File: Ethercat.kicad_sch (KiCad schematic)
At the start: 51 parts, among them J1 RJ45_Amphenol_RJMG1BD3B8K1ANR, J2 RJ45_Amphenol_RJMG1BD3B8K1ANR, Y1 25Mhz

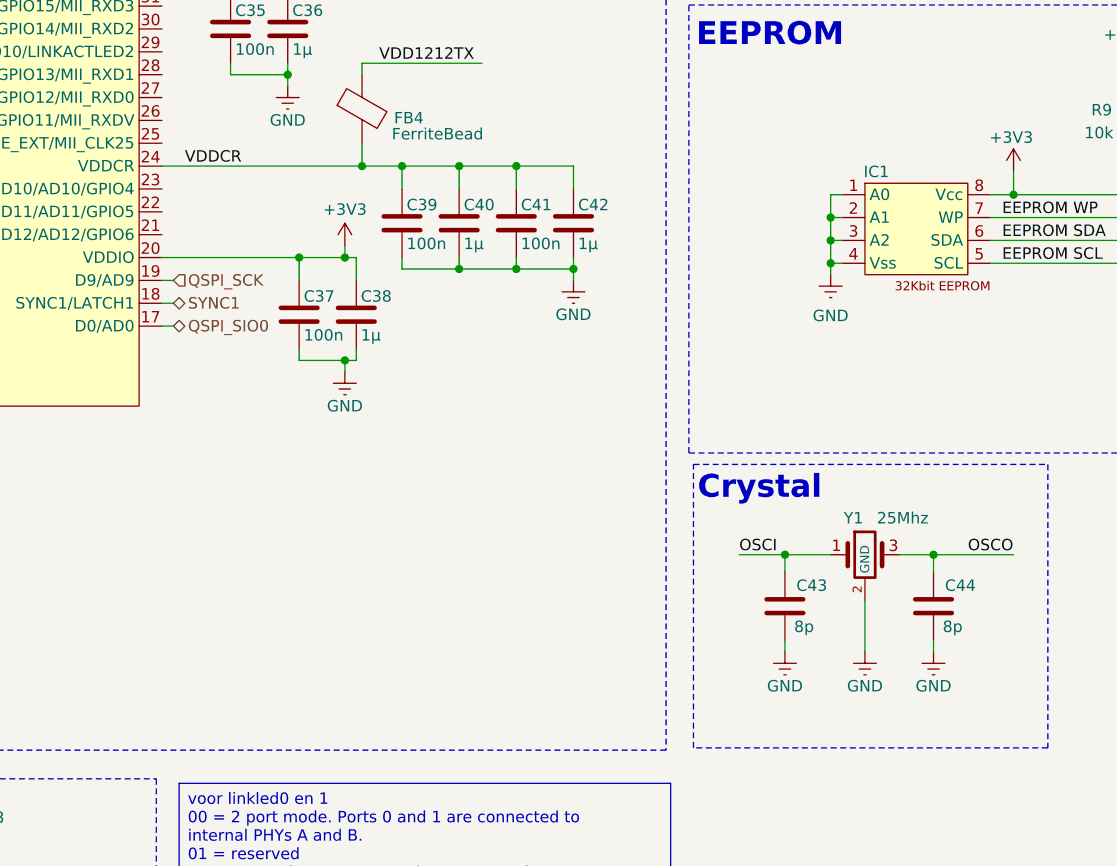
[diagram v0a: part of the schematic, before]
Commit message: al de main blokken bij elkaar gezet op juiste plaats
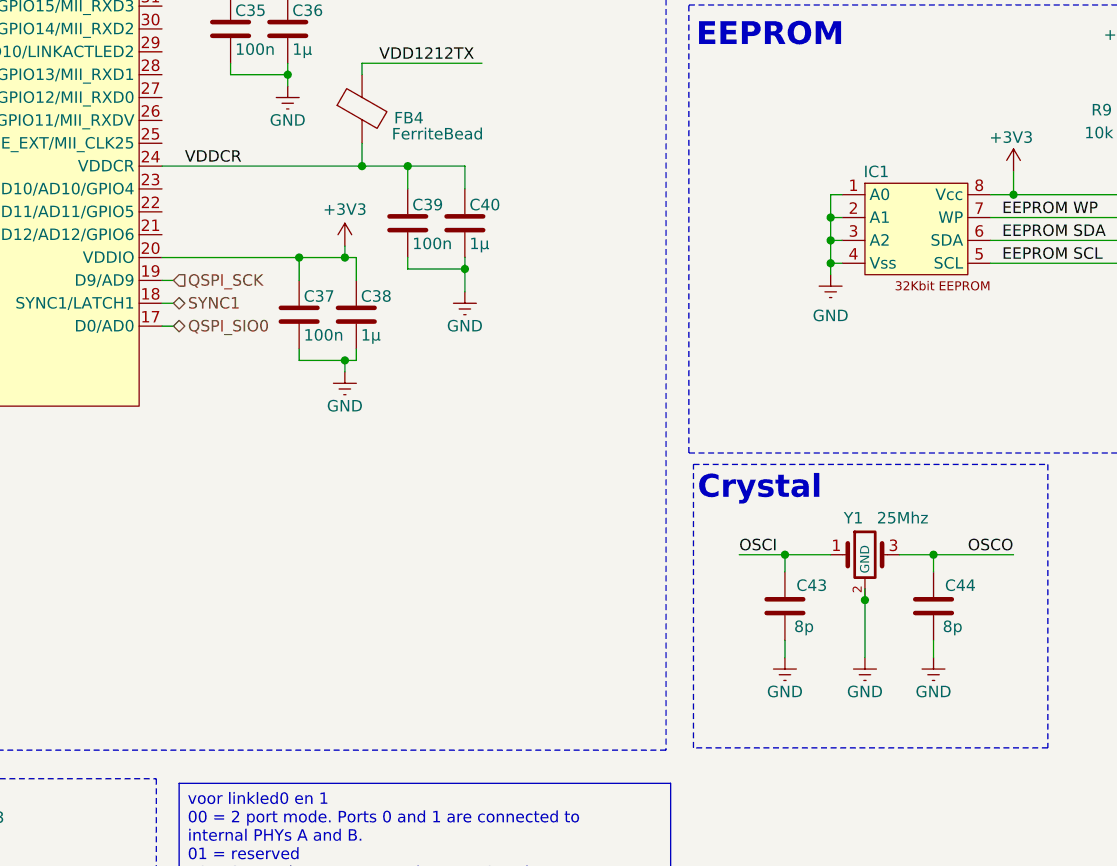
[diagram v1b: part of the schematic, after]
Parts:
- removed C41: 100n, Capacitor_SMD:C_0603_1608Metric, symbol Device:C
- removed C42: 1µ, Capacitor_SMD:C_0603_1608Metric, symbol Device:C
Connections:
- net GND: now also Y1.4 (GND); no longer Y1.2 (GND)
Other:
- moved on the sheet: C39, C40
